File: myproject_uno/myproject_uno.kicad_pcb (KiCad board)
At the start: 2 copper layers, 68.6 x 63.4 mm, 24 parts, among them J1 Conn_Coaxial, J2 Conn_01x03, J3 Conn_01x03, P1 Power, P2 Analog, P3 Digital, P4 Digital, U1 LTC1050, U2 RN2483, U3 LTC1050, U4 GazSensor

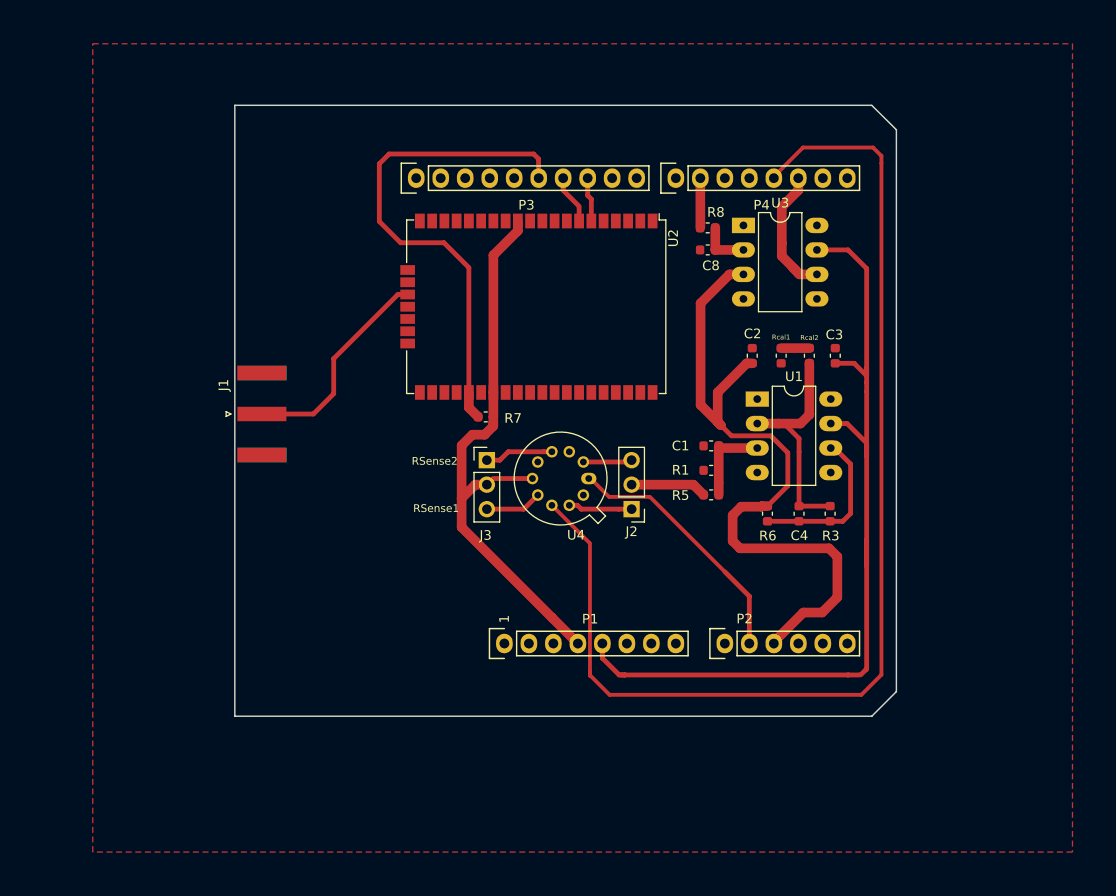
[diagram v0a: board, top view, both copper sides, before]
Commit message: final version
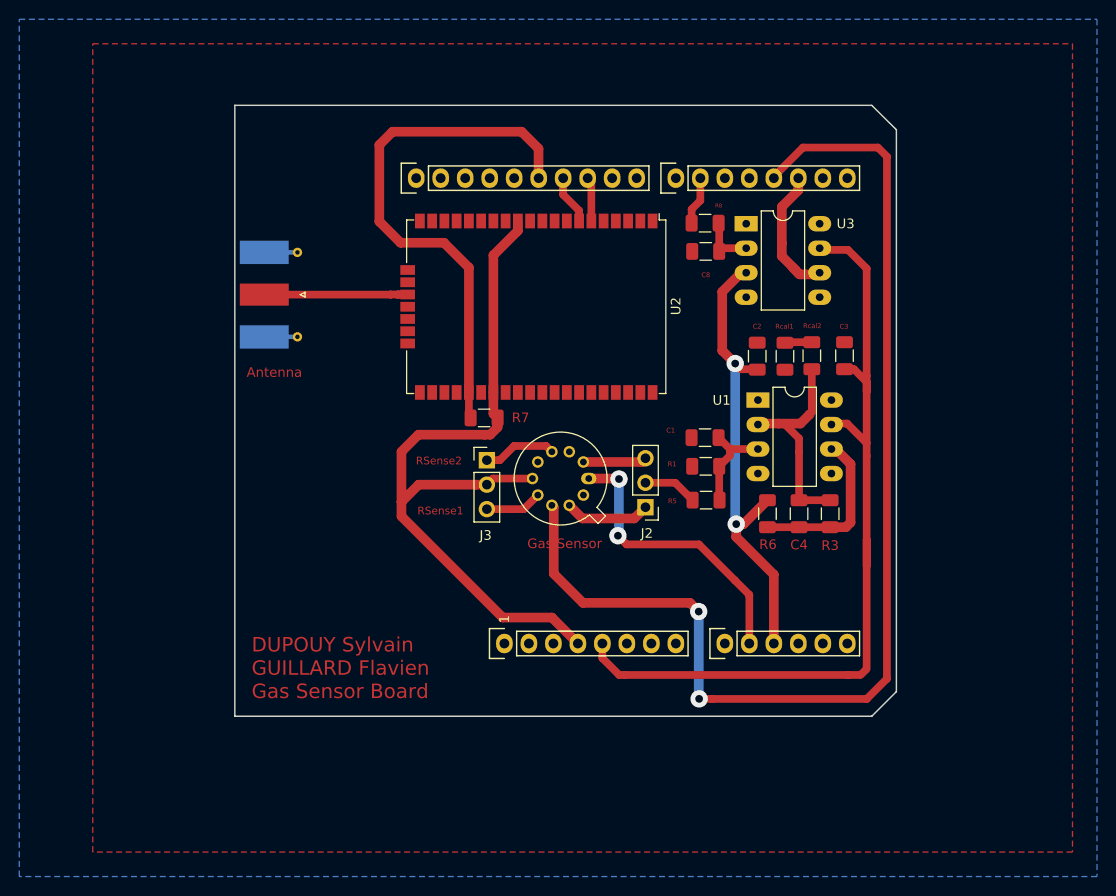
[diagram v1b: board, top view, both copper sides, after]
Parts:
- removed J1: Conn_Coaxial, Connector_Coaxial:SMA_Amphenol_132289_EdgeMount
- added Antenna: Conn_Coaxial, Connector_Coaxial:SMA_Molex_73251-1153_EdgeMount_Horizontal, F.Cu at (116.0, 89.5)
- C1, C2, C3, C4, C8: footprint Capacitor_SMD:C_0603_1608Metric -> Capacitor_SMD:C_1206_3216Metric
- Gas Sensor: renamed from U4
- R1, R3, R5, R6, R7, R8, Rcal1, Rcal2: footprint Resistor_SMD:R_0603_1608Metric -> Resistor_SMD:R_1206_3216Metric
- moved J2 1.45 mm to (153.8, 111.6)
- moved C1 1.06 mm to (160.0, 104.3)
- moved C3 0.96 mm to (174.5, 95.8)
- moved R5 0.76 mm to (160.1, 110.8)
- moved R1 0.70 mm to (160.1, 107.3)
- moved R8 0.56 mm to (160.0, 82.1)
- moved C2 0.52 mm to (165.4, 95.9)
- moved Rcal1 0.40 mm to (168.3, 95.9)
- moved U3 0.33 mm to (164.3, 82.2)
- moved C8 0.26 mm to (160.1, 85.0)
- moved Rcal2 0.26 mm to (171.1, 95.8)
- moved R7 0.20 mm to (137.1, 102.3)
- moved U1 0.12 mm to (165.5, 100.4)
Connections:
- U2 pad 23: Net-(J1-Pad1) -> ANT
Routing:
- net ANxArduino: track 73.6 -> 48.1 mm, vias 0 -> 2
- net Net-(J1-Pad1): track 22.4 -> 0.00 mm
- net +3V3: track 60.4 -> 78.8 mm
- net ANT: track 0.00 -> 15.9 mm
- net CapTemp: track 26.8 -> 30.6 mm, vias 0 -> 2
- net !RST: track 52.3 -> 55.7 mm
- net RChauff: track 118.2 -> 120.9 mm, vias 0 -> 2
- net Net-(J2-Pad1): track 6.63 -> 8.95 mm
- net Rsensor: track 7.90 -> 5.63 mm
- net Net-(C4-Pad1): track 24.9 -> 23.2 mm
- net Net-(J2-Pad3): track 5.08 -> 6.60 mm
- net Net-(C1-Pad1): track 9.97 -> 11.1 mm
- net +5V: track 92.7 -> 91.7 mm
- net Net-(C8-Pad1): track 5.21 -> 5.81 mm
- net RX: track 4.61 -> 5.13 mm
- added copper zone on B.Cu, net GND
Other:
- board text added: "DUPOUY Sylvain GUILLARD Flavien Gas Sensor Board"
